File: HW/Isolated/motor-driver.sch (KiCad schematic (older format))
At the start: 42 parts

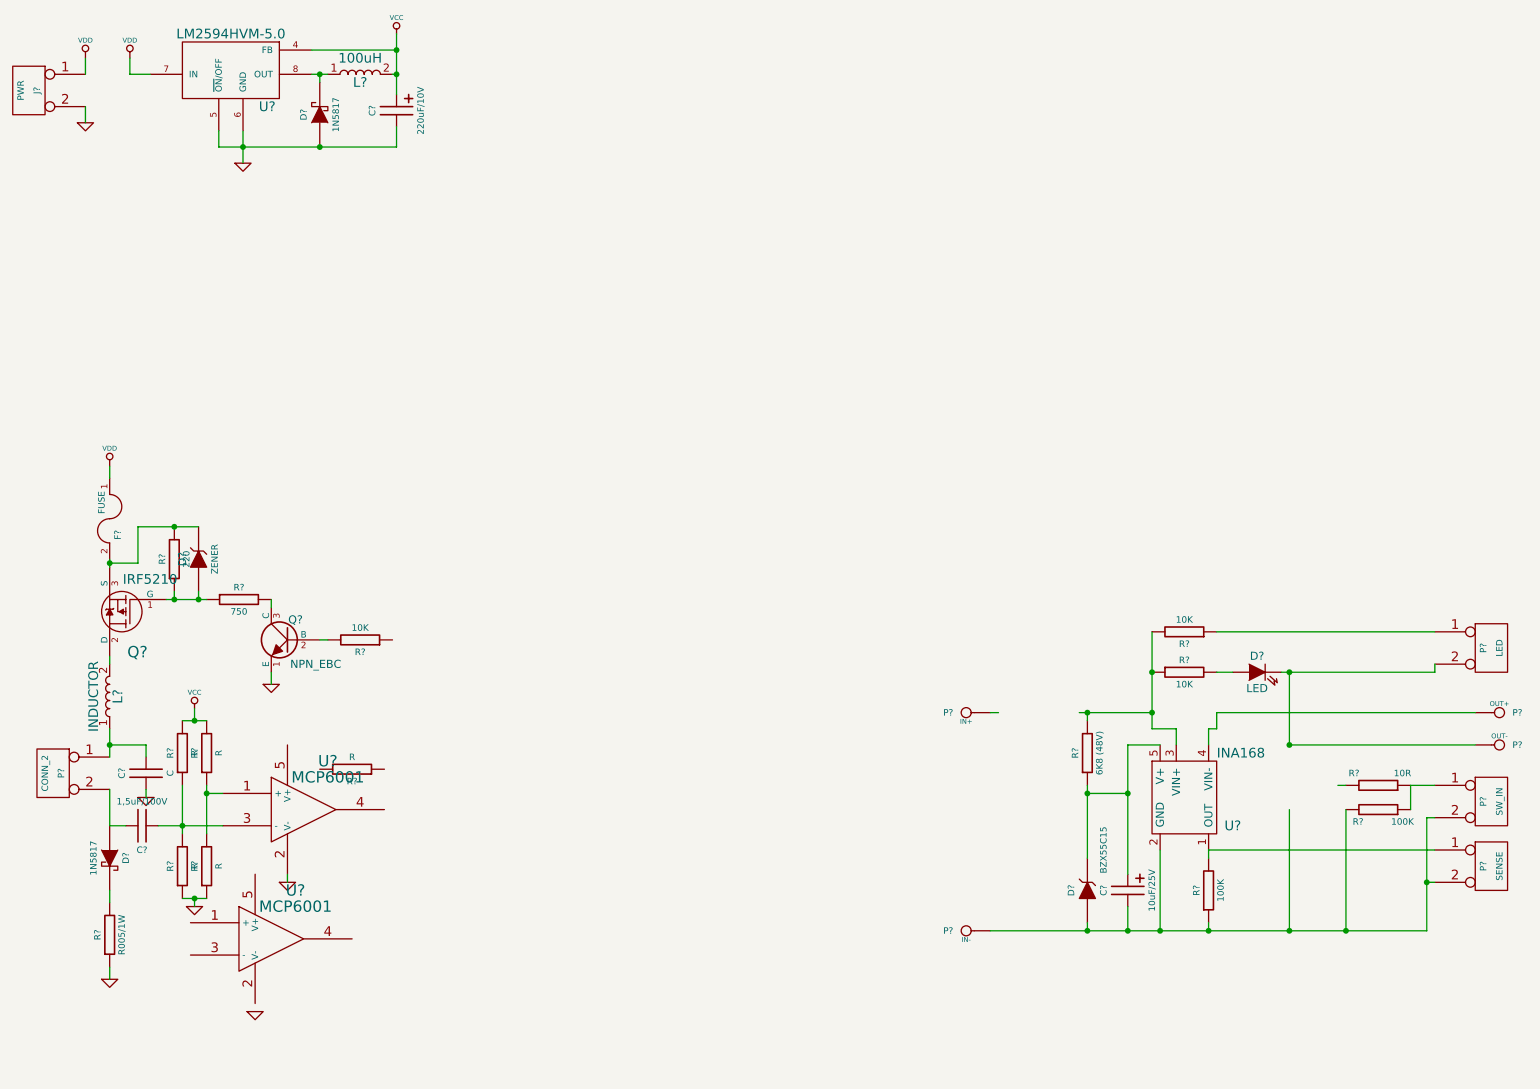
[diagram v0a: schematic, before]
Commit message: Schematic changed
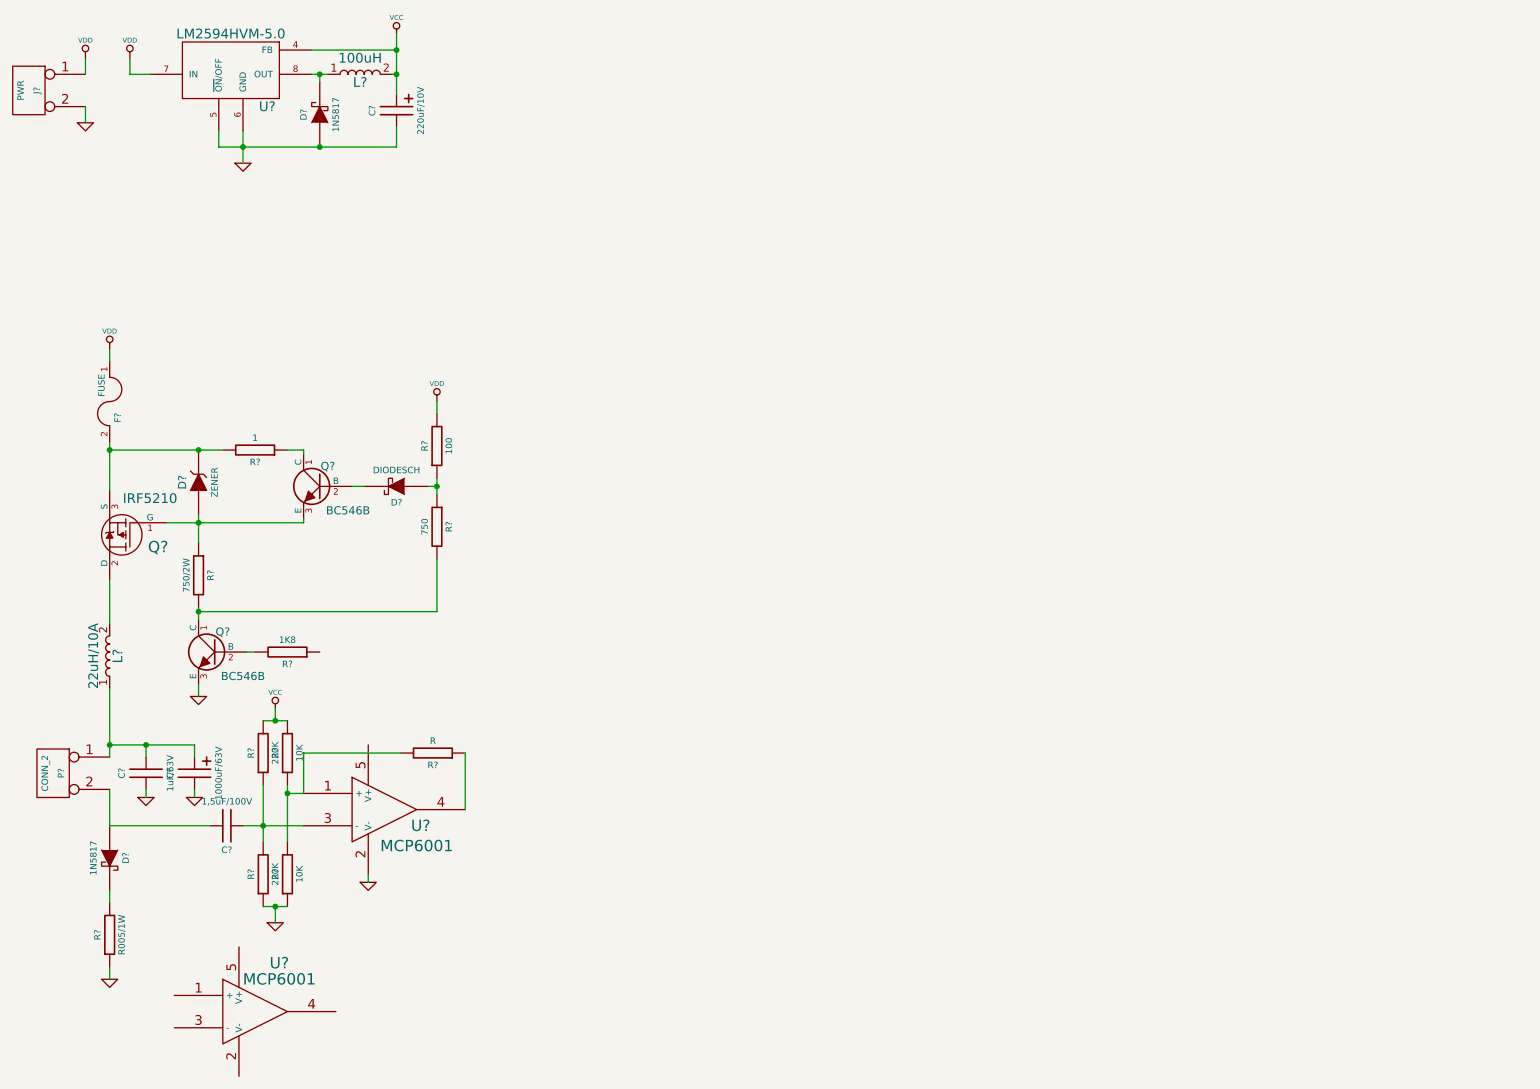
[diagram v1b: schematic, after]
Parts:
- removed C?: 10uF/25V, C1P_D2, symbol CP
- removed D?: LED, LED3, symbol LED
- removed D?: BZX55C15, D3, symbol ZENER
- removed P?: IN+, HEADER_6.3, symbol CONN_1
- removed P?: OUT+, HEADER_6.3, symbol CONN_1
- removed P?: OUT-, HEADER_6.3, symbol CONN_1
- removed P?: IN-, HEADER_6.3, symbol CONN_1
- removed P?: LED, HDR-2, symbol CONN_2
- removed P?: SW_IN, HDR-2, symbol CONN_2
- removed P?: SENSE, HDR-2, symbol CONN_2
- removed Q?: NPN_EBC, ~, symbol NPN_EBC
- removed R?: 10R, R4, symbol R
- removed R? (x2): 100K, R4, symbol R
- removed R? (x2): 10K, R4, symbol R
- removed R?: 6K8 (48V), R4, symbol R
- removed R?: 220, ~, symbol R
- removed U?: INA168, SOT23-5, symbol INA168
- added C?: 1000uF/63V, ~, symbol CP
- added D?: DIODESCH, symbol DIODESCH
- added Q? (x2): BC546B, TO-92, symbol NPN_CBE
- added R?: 1, R4, symbol R
- added R?: 750, R6, symbol R
- added R?: 100, R4, symbol R
- C?: value C -> 1uF/63V
- L?: value INDUCTOR -> 22uH/10A
- R? (x2): value R -> 220K; footprint ~ -> R4
- R? (x2): value R -> 10K; footprint ~ -> R4
- R?: value 750 -> 750/2W; footprint ~ -> R6
- R?: value 10K -> 1K8; footprint ~ -> R4
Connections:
- wire segments 77 -> 53
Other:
- moved on the sheet: C?, D?, F?, L?, Q?, R?, U?
